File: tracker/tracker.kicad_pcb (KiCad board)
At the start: 4 copper layers, 49.4 x 53.2 mm, 86 parts, among them J1 Conn_01x05, J2 SIM_Card, J3 Conn_01x01, J4 Conn_01x01, J5 Conn_Coaxial, J6 Conn_01x02, M1 BG96, Q2 DMP2008UFG, U1 STM32U545CEUx, U10 PUMH10,115, U11 PUMH10,115, U12 DF6A6.8FUT, U2 GD25QxxxEY, U3 NXB0108PW, U4 AP22800HB-7, U6 LMR51430, U7 AP61100Z6, U8 PUMH10,115, Y2 8MHz, Y3 32.768KHz

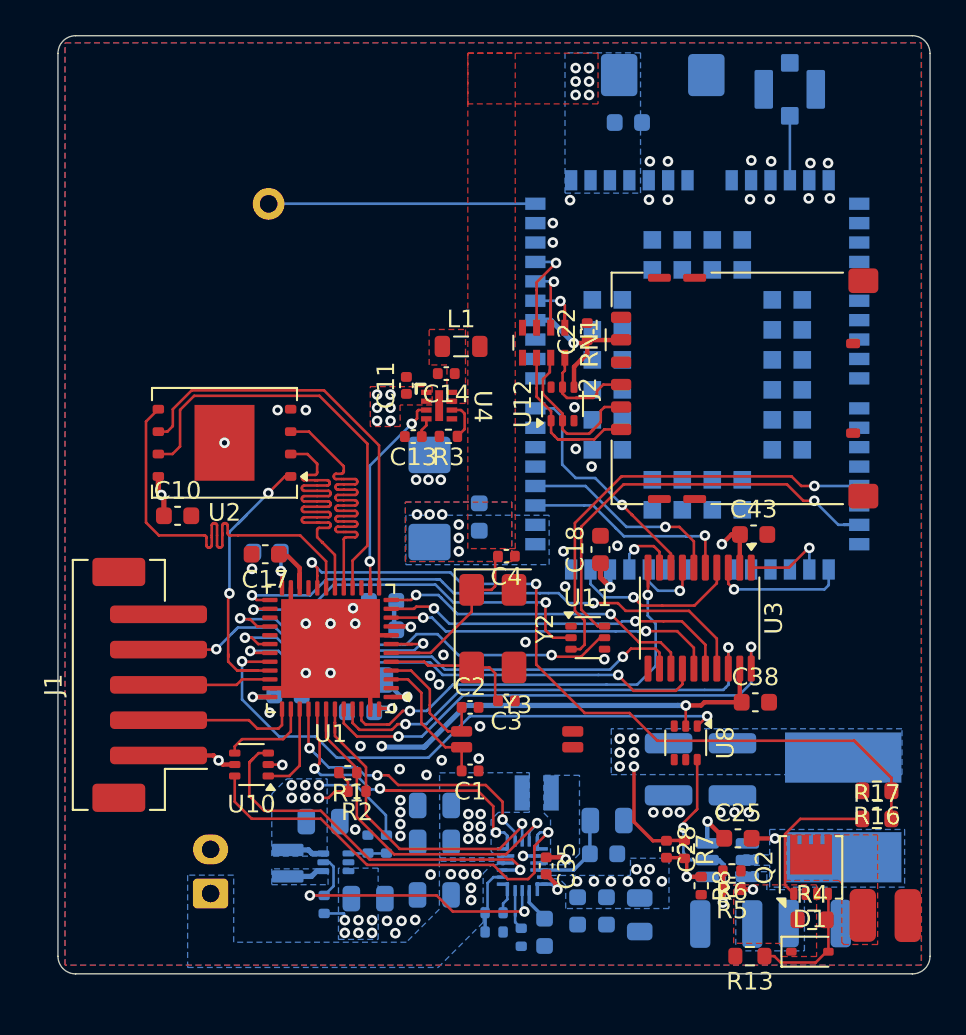
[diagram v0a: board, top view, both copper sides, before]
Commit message: save
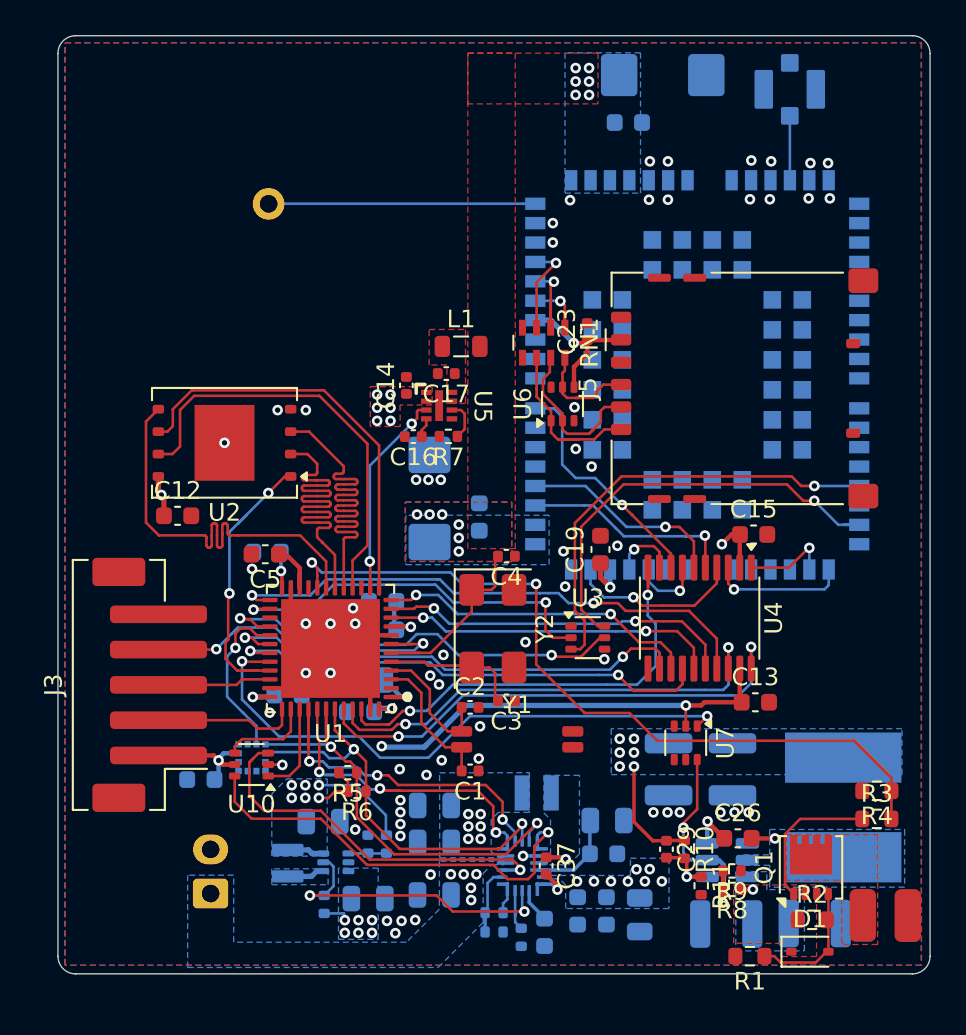
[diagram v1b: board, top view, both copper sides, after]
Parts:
- added C42: 0.1u, Capacitor_SMD:C_0603_1608Metric, B.Cu at (130.7, 85.5)
- added U12: MC3479, Package_LGA:LGA-12_2x2mm_P0.5mm, B.Cu at (133.6, 84.3)
- renumbered C8 to C10, C9 to C11, C10 to C12, C38 to C13, C11 to C14, C43 to C15, C13 to C16, C14 to C17, C15 to C18, C18 to C19, C16 to C20, C20 to C21, C21 to C22, C22 to C23, C23 to C24, C24 to C25, C25 to C26, C26 to C27, C27 to C28, C28 to C29, C29 to C30, C30 to C31, C31 to C32, C32 to C33, C41 to C34, C33 to C35, C42 to C36, C35 to C37, C36 to C38, C37 to C39, C39 to C40, C40 to C41, C17 to C5, C5 to C6, C19 to C7, C6 to C8, C7 to C9, J3 to J1, J4 to J2, J1 to J3, J5 to J4, J2 to J5, Q2 to Q1, R13 to R1, R7 to R10, R8 to R11, R14 to R12, R9 to R13, R10 to R14, R11 to R16, R12 to R17, R4 to R2, R17 to R3, R16 to R4, R1 to R5, R2 to R6, R3 to R7, R5 to R8, R6 to R9, U9 to U11, U11 to U3, U3 to U4, U4 to U5, U12 to U6, U8 to U7, U6 to U8, U7 to U9, Y3 to Y1
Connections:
- net /mcu/I2C_SCL renamed /I2C_SCL
- net /mcu/I2C_SDA renamed /I2C_SDA
- U1 pad 29: unconnected-(U1-PA8-Pad29) -> /accelerometer/ACC_INT1
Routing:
- net /accelerometer/ACC_INT1: track 0.00 -> 9.39 mm, vias 0 -> 1
- net /I2C_SDA: track 18.7 -> 23.5 mm, vias 1 -> 2
- net /I2C_SCL: track 21.4 -> 25.3 mm, vias 1 -> 2
- net +3V3: track 55.5 -> 58.1 mm
- net /battery charger/CHARGER_INT: track 17.1 -> 19.6 mm
- net /battery charger/CHARGER_STAT: track 18.1 -> 18.7 mm
- net GND: vias 63 -> 62
